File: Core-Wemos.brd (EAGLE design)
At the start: 99.8 x 80.5 mm, 23 parts, among them IC1 7805, J3 CONNECTOR-GROVE-4P-2.0-347013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

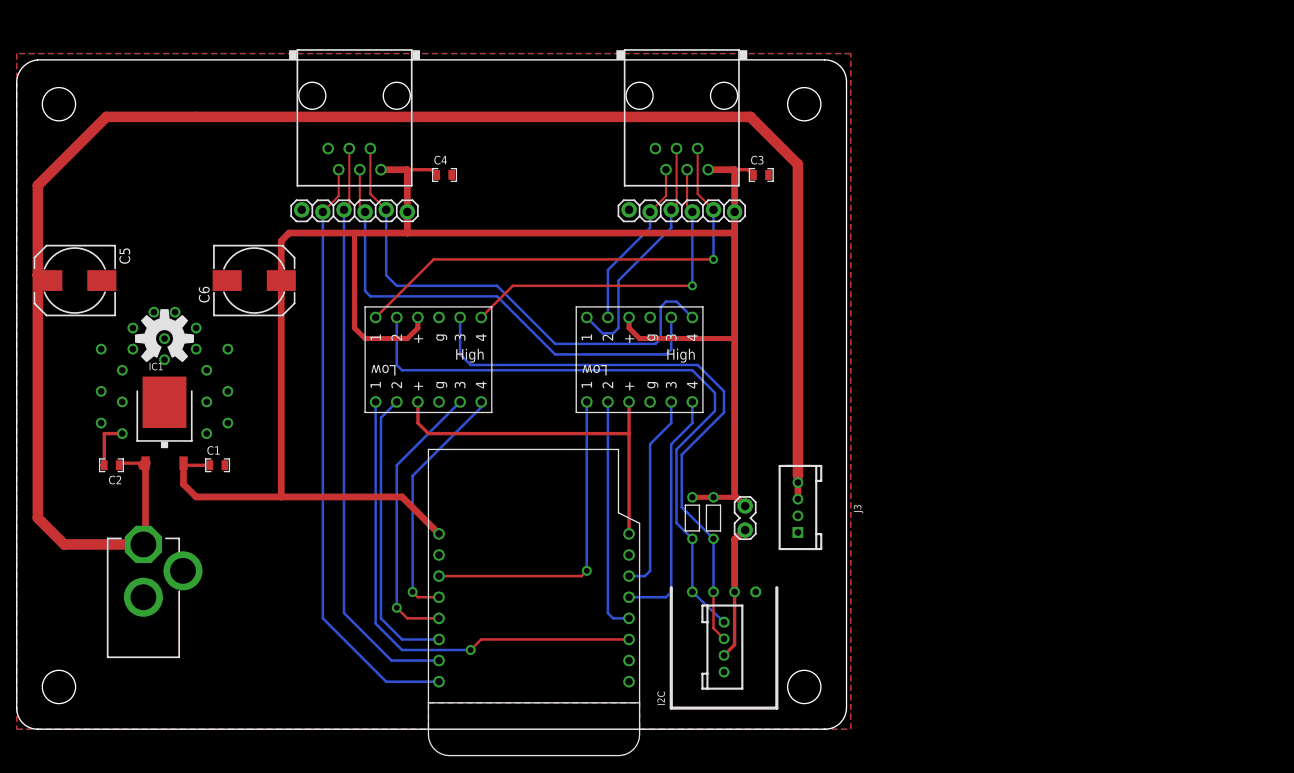
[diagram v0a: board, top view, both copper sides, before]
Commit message: 2.0
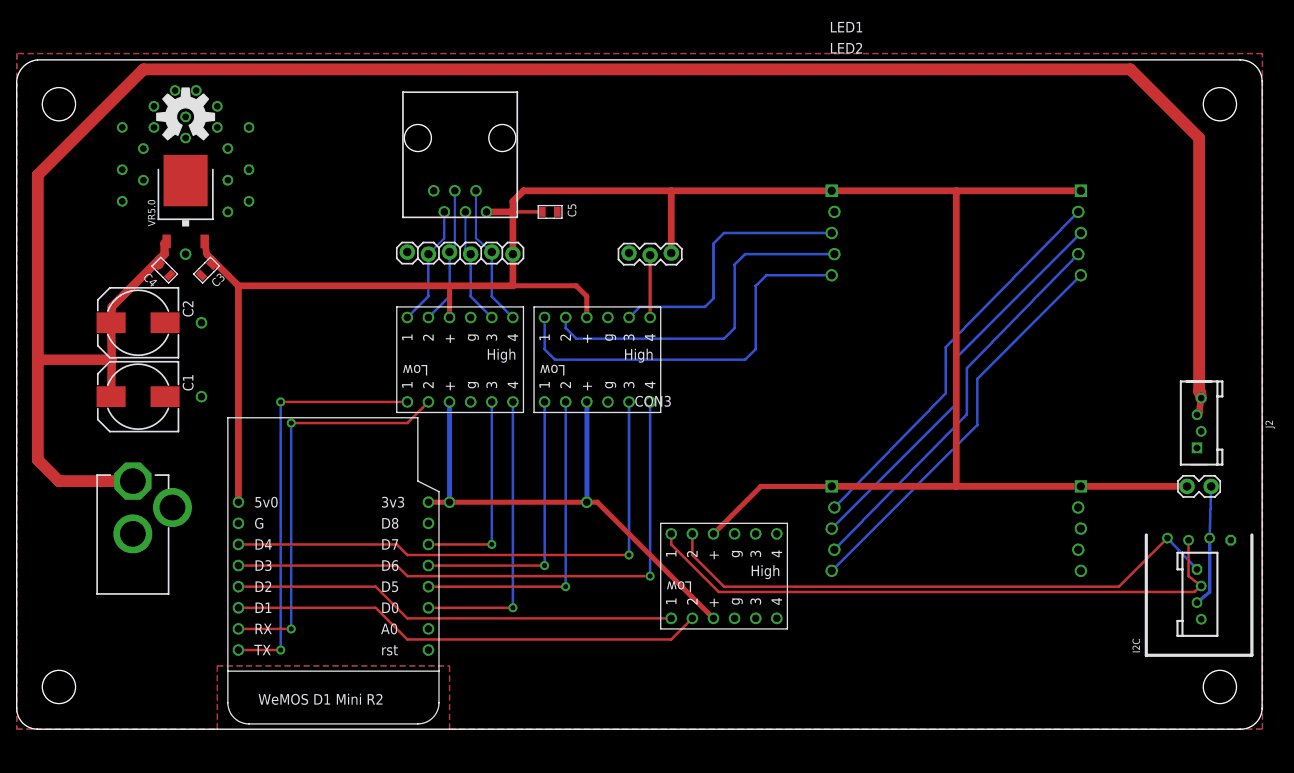
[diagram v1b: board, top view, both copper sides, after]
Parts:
- removed C6: 150uF, SPCoast:0810-CAP
- removed IC1: 7805, SPCoast:TO252
- removed J4: (no value), SPCoast:DCJ0202
- removed J5: (no value), SPCoast:RJ25
- removed JP10, JP11: (no value), SparkFun-Connectors:1X06_LOCK
- removed JP5: 5v I2C Power, SparkFun-Connectors:1X02_LOCK
- removed R101, R111: 1k8, SPCoast:1/6W-RES
- removed U$1: OSHW-LOGOL, SparkFun:OSHW-LOGO-L
- removed U$2: (no value), SPCoast:WEMOS-D1
- removed U$3: 9-12vDC, SPCoast-minimal:POWER_USAGE
- removed U$4: BOARD80X100, SPCoast:BOARD-DINRAIL-3.17IN
- removed U$5, U$6: VMATCH, SPCoast:VMATCH
- added BOARD: BOARD80X150, SPCoast:BOARD-DINRAIL-3.17INX15CM
- added CON3: (no value), SPCoast:1X03
- added J1: (no value), SPCoast:DCJ0202
- added JP2: 5v I2C Power, SparkFun-Connectors:1X02_LOCK
- added JP3: (no value), SparkFun-Connectors:1X06_LOCK
- added LABEL1: 7-12vDC, SPCoast-minimal:POWER_USAGE
- added LED1, LED2: LEDMATRIX, SPCoast:LEDMATRIX
- added LS1, LS2, LS3: (no value), SPCoast:MODULE
- added OSHW1: OSHW-LOGOL, SparkFun:OSHW-LOGO-L
- added VR5.0: 5v, SPCoast:TO-252
- added WEMOS: D1Mini, SPCoast:WEMOS-D1
- C1, C2: value 1uF -> 150uF; device SPCoast:0805-CAP -> SPCoast:0810-CAP
- C3, C4: value 1uF -> 0.1uF
- C5: value 150uF -> 0.1uF; device SPCoast:0810-CAP -> SPCoast:0805-CAP
- J2: value (none) -> CONNECTOR-GROVE-4P-2.0-3470130P1; device SPCoast:RJ25 -> SPCoast:4P-2.0
- J3: value CONNECTOR-GROVE-4P-2.0-3470130P1 -> (none); device SPCoast:4P-2.0 -> SPCoast:RJ25-TOP
- moved J2 73.6 mm to (142.2, 36.8), turned to 90 degrees
- moved C3 67.6 mm to (22.9, 55.2), turned to 225 degrees
- moved J3 60.2 mm to (53.3, 71.1), turned to 180 degrees
- moved C5 57.7 mm to (64.1, 62.2), turned to 0 degrees
- moved I2C 57.5 mm to (142.2, 22.9)
- moved C4 35.5 mm to (17.8, 55.2), turned to 315 degrees
- moved C2 17.4 mm to (14.6, 48.9)
- moved C1 12.6 mm to (14.6, 40.0), turned to 180 degrees
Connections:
- removed net +3V3: U$2.3V3, U$5.LV, U$6.LV
- removed net A0: U$2.A0
- removed net D8: U$2.D8
- new net 3V3: LS1.LV, LS2.LV, LS3.LV, WEMOS.3V3
- new net N$10: LED1.CLK@2, LED2.CLK@1
- new net N$3: LED1.DO, LED2.DI
- new net N$9: LED1.CS@2, LED2.CS@1
- new net RXH: J3.4, JP3.4, LS1.H2
- new net TXH: J3.5, JP3.5, LS1.H1
- net +9V: now also C1.+, C2.+, C4.1, J1.1, J2.3, J2.4, VR5.0.1; no longer C2.1, C5.+, IC1.1, J3.3, J3.4, J4.1
- net D0: now also LS1.L4, WEMOS.D0; no longer U$2.D0, U$6.L1
- net D0H: now also J3.2, JP3.2, LS1.H4; no longer J2.2, JP10.2, U$6.H1
- net D3: now also LS2.L4, WEMOS.D3; no longer U$2.D3, U$6.L4
- net D3H: now also CON3.2, LS2.H4; no longer J2.3, JP10.3, U$6.H4
- net D4: now also LS2.L3, WEMOS.D4; no longer U$2.D4, U$5.L1
- net D4H: now also LED1.DI, LS2.H3; no longer J2.4, JP10.4, U$5.H1
- net D5: now also LS2.L2, WEMOS.D5; no longer U$2.D5, U$5.L2
- net D5H: now also LED1.CS@1, LS2.H2; no longer J2.5, JP10.5, U$5.H2
- net D6: now also LS2.L1, WEMOS.D6; no longer U$2.D6, U$5.L4
- net D6H: now also LED1.CLK@1, LS2.H1; no longer J5.2, JP11.2, U$5.H4
- net D7: now also LS1.L3, WEMOS.D7; no longer U$2.D7, U$5.L3
- net D7H: now also J3.3, JP3.3, LS1.H3; no longer J5.3, JP11.3, U$5.H3
- net GND: now also C1.-, C2.-, C5.2, CON3.3, J1.2, J1.3, J2.1, J2.2, J3.6, JP3.6, LED1.G@1, LED1.G@2, LED2.G@1, LED2.G@2, LS1.GND@0, LS1.GND@1, LS2.GND@0, LS2.GND@1, LS3.GND@0, LS3.GND@1, VR5.0.2, WEMOS.GND; no longer C1.2, C2.2, C5.-, C6.-, IC1.2, J2.6, J3.1, J3.2, J4.2, J4.3, J5.6, JP10.6, JP11.6, U$2.GND, U$5.GND@0, U$5.GND@1, U$6.GND@0, U$6.GND@1
- net N$44: now also JP2.1; no longer JP5.1
- net RX: now also LS1.L2, WEMOS.RX; no longer J5.4, JP11.4, U$2.RX
- net SCL: now also LS3.L2, WEMOS.D1; no longer U$2.D1, U$6.L2
- net SCLH: now also LS3.H2; no longer R111.2, U$6.H2
- net SDA: now also LS3.L1, WEMOS.D2; no longer U$2.D2, U$6.L3
- net SDAH: now also LS3.H1; no longer R101.2, U$6.H3
- net TX: now also LS1.L1, WEMOS.TX; no longer J5.5, JP11.5, U$2.TX
- net VCCIO: now also C5.1, CON3.1, J3.1, JP2.2, JP3.1, LED1.V+@1, LED1.V+@2, LED2.V+@1, LED2.V+@2, LS1.HV, LS2.HV, LS3.HV, VR5.0.3, WEMOS.5V; no longer C1.1, C4.1, C6.+, IC1.3, J2.1, J5.1, JP10.1, JP11.1, JP5.2, R101.1, R111.1, U$2.5V, U$5.HV, U$6.HV
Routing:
- net 3V3: track 0.00 -> 64.2 mm, vias 0 -> 2
- net +9V: track 208.4 -> 259.6 mm
- net N$10: track 0.00 -> 48.0 mm
- net N$3: track 0.00 -> 48.0 mm
- net N$9: track 0.00 -> 47.5 mm
- net D7H: track 58.9 -> 14.0 mm
- net +3V3: track 44.3 -> 0.00 mm
- net VCCIO: track 227.3 -> 271.5 mm
- net D3: track 29.7 -> 71.0 mm
- net GND: track 6.35 -> 47.5 mm, vias 20 -> 22
- net D0H: track 57.7 -> 17.2 mm, vias 1 -> 0
- net D3H: track 41.2 -> 7.49 mm, vias 1 -> 0
- net D4: track 38.4 -> 65.9 mm
- net D0: track 59.0 -> 34.9 mm
- net D5H: track 20.7 -> 43.4 mm
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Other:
- board size 99.8 x 80.5 mm -> 149.8 x 80.5 mm
- board text added: "2016.12"
- board text added: "5V I/O"
- board text added: "CS D5"
- board text added: "Clock D6"
- board text added: "Codeline"
- board text added: "Core WeMos"
- board text added: "D1 SCL"
- board text added: "D2 SDA"
- board text added: "Data D4"
- board text added: "IO4 breakout, I2C master and Codeline Matrix"
- board text added: "WeMOS D1 Mini R2"
- board text added: "v2.0"
- board text removed: "1k8"
- board text removed: "2016.10"
- board text removed: "3.3v"
- board text removed: "Core WeMOS D1"
- board text removed: "D1"
- board text removed: "D2"
- board text removed: "I2C Term"
- board text removed: "IO4 breakout and I2C baseboard"
- board text removed: "SCL"
- board text removed: "SDA"
- board text removed: "v1.0"
